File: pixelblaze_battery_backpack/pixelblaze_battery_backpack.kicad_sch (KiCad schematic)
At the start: 45 parts, among them J1 Conn_01x01, J10 Conn_01x04, J11 Conn_01x04, J12 Conn_01x08, J13 Conn_01x04, J14 Conn_01x04, J15 Conn_01x04, J2 Conn_01x01, J3 Conn_01x01, J4 Conn_01x01, J5 USB_C_Receptacle_USB2.0_16P, J6 Conn_ARM_SWD_TagConnect_TC2030, J7 Conn_01x04, J8 Conn_QWIIC_Horizontal, J9 Conn_01x04, U1 HUSB238, U2 MSPM0C110xSRUK, U3 BQ25798, U4 LIS3DH, U6 AP2112K-3.3

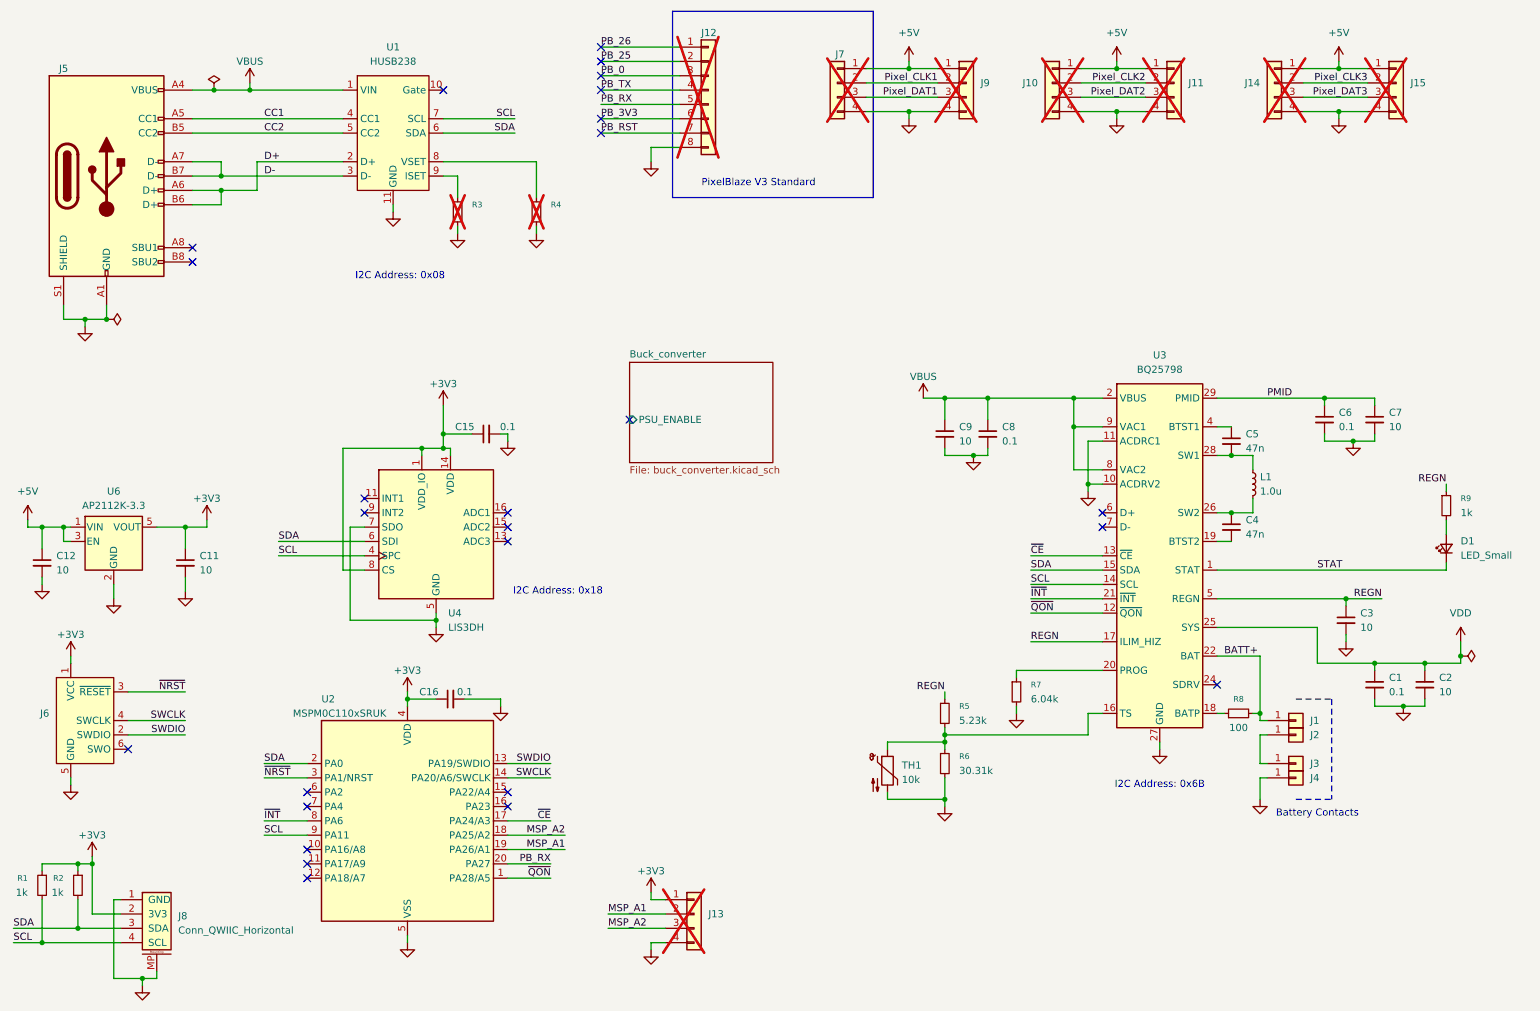
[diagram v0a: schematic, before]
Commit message: Checkpoint, changing computers
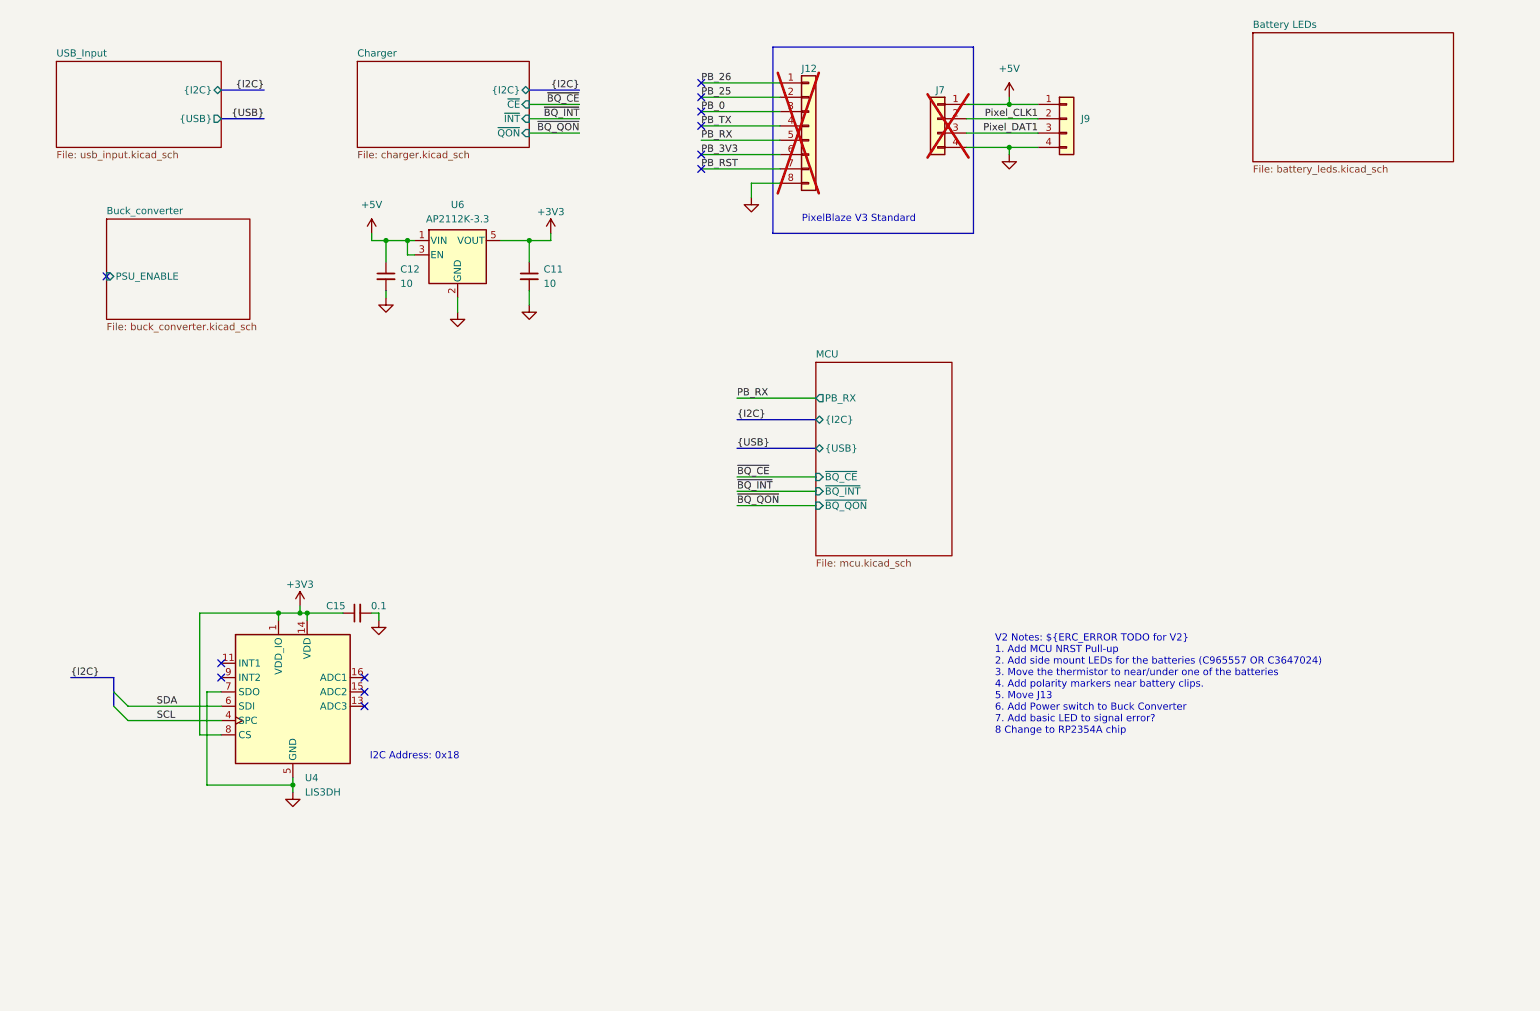
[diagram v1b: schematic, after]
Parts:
- removed C1, C16, C6, C8: 0.1, Capacitor_SMD:C_0402_1005Metric, symbol Device:C_Small
- removed C2, C3, C7, C9: 10, Capacitor_SMD:C_0603_1608Metric, symbol Device:C_Small
- removed C4, C5: 47n, Capacitor_SMD:C_0402_1005Metric, symbol Device:C_Small
- removed D1: LED_Small, LED_SMD:LED_0603_1608Metric, symbol Device:LED_Small
- removed J1, J2, J3, J4: Conn_01x01, Battery:BatteryClip_MYoung_MY-18650-01, symbol Connector_Generic:Conn_01x01
- removed J10, J11, J13, J14, J15: Conn_01x04, Connector_PinHeader_2.54mm:PinHeader_1x04_P2.54mm_Vertical, symbol Connector_Generic:Conn_01x04
- removed J5: USB_C_Receptacle_USB2.0_16P, Connector_USB:USB_C_Receptacle_HRO_TYPE-C-31-M-12, symbol Connector:USB_C_Receptacle_USB2.0_16P
- removed J6: Conn_ARM_SWD_TagConnect_TC2030, Connector:Tag-Connect_TC2030-IDC-FP_2x03_P1.27mm_Vertical, symbol Connector:Conn_ARM_SWD_TagConnect_TC2030
- removed J8: Conn_QWIIC_Horizontal, Connector_JST:JST_SH_SM04B-SRSS-TB_1x04-1MP_P1.00mm_Horizontal, symbol SKEC_Symbols:Conn_QWIIC_Horizontal
- removed L1: 1.0u, Inductor_SMD:L_Changjiang_FXL0630, symbol Device:L_Small
- removed R1, R2, R9: 1k, Resistor_SMD:R_0402_1005Metric, symbol Device:R_Small
- removed R3, R4: R_Small, Resistor_SMD:R_0402_1005Metric, symbol Device:R_Small
- removed R5: 5.23k, Resistor_SMD:R_0402_1005Metric, symbol Device:R_Small
- removed R6: 30.31k, Resistor_SMD:R_0402_1005Metric, symbol Device:R_Small
- removed R7: 6.04k, Resistor_SMD:R_0402_1005Metric, symbol Device:R_Small
- removed R8: 100, Resistor_SMD:R_0402_1005Metric, symbol Device:R_Small
- removed TH1: 10k, Resistor_SMD:R_0603_1608Metric, symbol Device:Thermistor_NTC
- removed U1: HUSB238, Package_DFN_QFN:DFN-10-1EP_3x3mm_P0.5mm_EP1.65x2.38mm_ThermalVias, symbol Interface_USB:HUSB238_002DD
- removed U2: MSPM0C110xSRUK, Package_DFN_QFN:Texas_RUK0020B_WQFN-20-1EP_3x3mm_P0.4mm_EP1.7x1.7mm_ThermalVias, symbol MCU_Texas:MSPM0C110xSRUK
- removed U3: BQ25798, Package_DFN_QFN:Texas_RQM0029A_VQFN-29_4x4mm_P0.4mm, symbol Battery_Management:BQ25798
- J9: footprint Connector_PinHeader_2.54mm:PinHeader_1x04_P2.54mm_Vertical -> Connector_Molex:Molex_Micro-Fit_3.0_43650-0415_1x04_P3.00mm_Vertical; JLCPCB Part No. (none) -> C293547; MPN (none) -> 436500415; now fitted
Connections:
- no-connect marks 26 -> 12
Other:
- added sheet Battery LEDs (battery_leds.kicad_sch)
- added sheet Charger (charger.kicad_sch)
- added sheet MCU (mcu.kicad_sch)
- added sheet USB_Input (usb_input.kicad_sch)
- note added: "V2 Notes: ${ERC_ERROR TODO for V2} 1. Add MCU NRST Pull-up 2. Add side mount LEDs for the batteries (C965557 OR C3647024) 3. Move the thermistor to near/under one of the batteries 4. Add polarity markers near battery clips. 5. Move J13 6. Add Power switch to Buck Converter 7. Add basic LED to signal error? 8 Change to RP2354A chip"
- note removed: "Battery Contacts"
- note removed: "I2C Address: 0x08"
- note removed: "I2C Address: 0x6B"
- moved on the sheet: C11, C12, C15, J12, J7, U4, U6
